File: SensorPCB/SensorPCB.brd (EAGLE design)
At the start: 36 x 66 mm, 31 parts, among them T1 33u

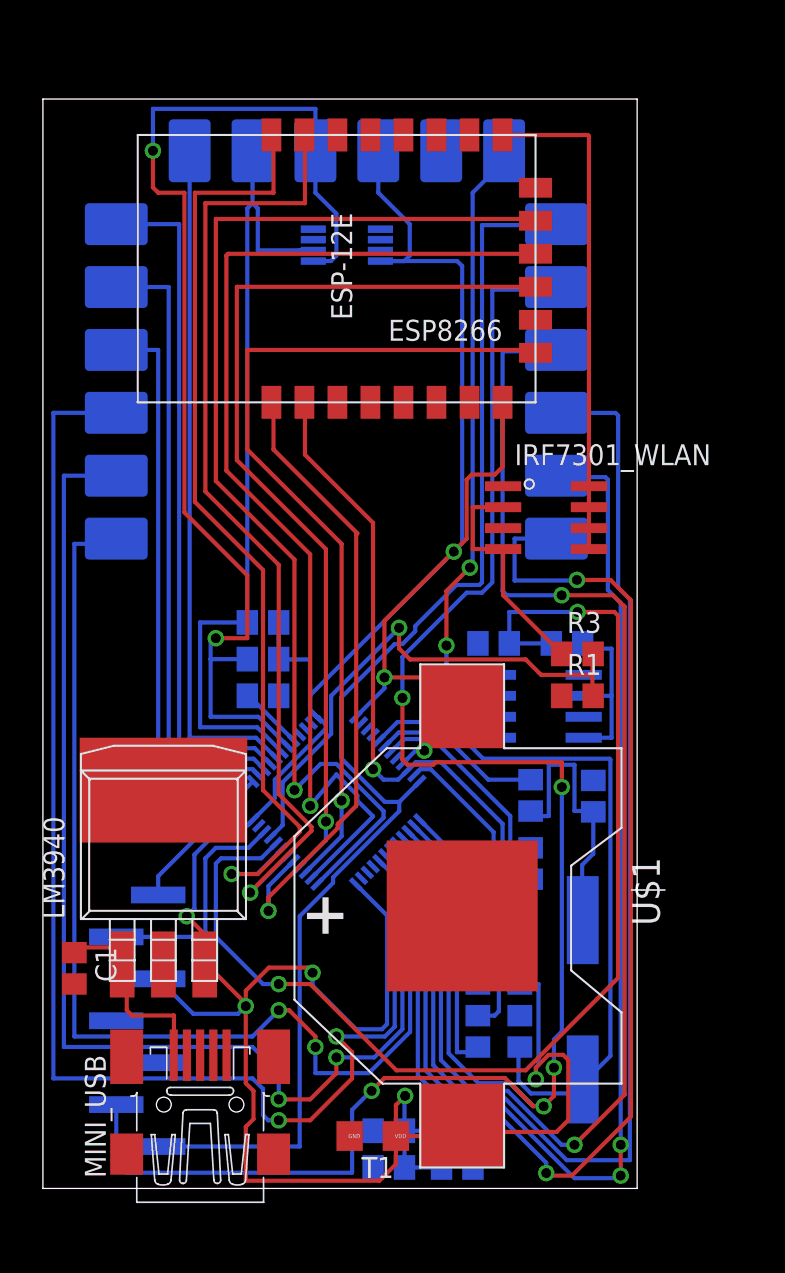
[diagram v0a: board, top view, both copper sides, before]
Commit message: start new board version
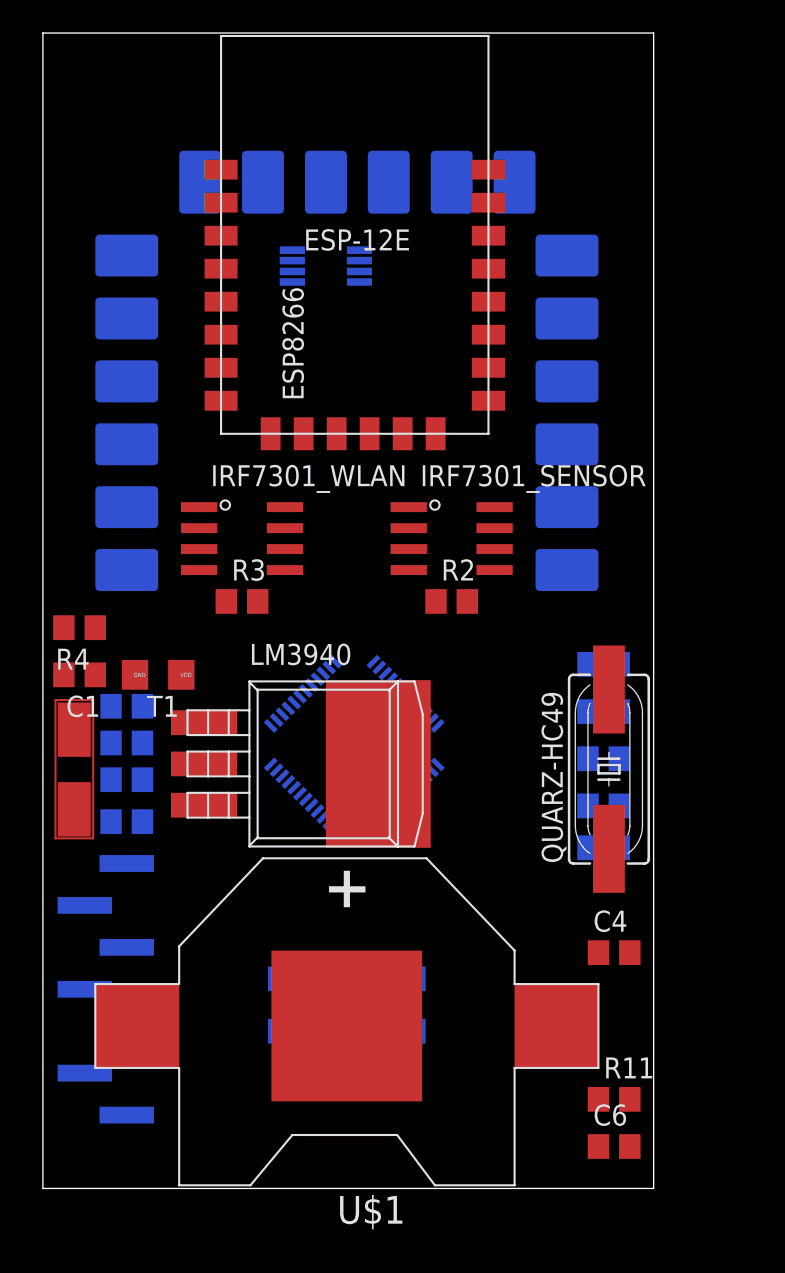
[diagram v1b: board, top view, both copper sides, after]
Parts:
- removed MINI_USB: MINI-USB-SCHIELD-32005-201, con-cypressindustries:32005-201
- added R4: 10k, rcl:R0805
- added U$2: 5V_POWER_SUPPLY, 5V_POWER_SUPPLY:5V_POWER_SUPPLY
- moved T1 30.8 mm to (6.99, 31.1)
- moved R1 27.8 mm to (5.08, 24.8), flipped to the bottom, turned to 180 degrees
- moved R6 24.7 mm to (5.08, 22.2)
- moved C6 21.3 mm to (34.6, 2.54), flipped to the top, turned to 0 degrees
- moved R10 20.9 mm to (34.0, 28.9)
- moved R3 20.6 mm to (12.1, 35.6)
- moved ESP8266 19.1 mm to (10.8, 45.7), turned to 0 degrees
- moved R11 19.1 mm to (34.6, 5.40), flipped to the top, turned to 0 degrees
- moved IRF7301_WLAN 18.5 mm to (12.1, 39.4)
- moved R7 18.2 mm to (34.0, 26.0), turned to 0 degrees
- moved C1 17.8 mm to (2.22, 31.1), turned to 180 degrees
- moved QUARZ-HC49 14.1 mm to (34.3, 25.4), flipped to the top, turned to 90 degrees
- moved C8 12.9 mm to (15.2, 9.53), turned to 0 degrees
- moved C10 12.9 mm to (34.0, 31.8), turned to 0 degrees
- moved C3 12.8 mm to (15.2, 12.7)
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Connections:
- removed net CH_PD_WLAN: ESP8266.3
- removed net D+: MINI_USB.3
- removed net D-: MINI_USB.2
- removed net ID: MINI_USB.4
- new net ADC: R7.2, R8.1, STM32L051C8T6.10
- new net CHPD: ESP8266.3, R4.1
- net +3V3: now also R4.2
- net +5V: now also U$2.MINUS; no longer MINI_USB.1
- net ADC_WLAN: no longer R7.2, R8.1, STM32L051C8T6.10
- net GND: now also U$2.PLUS; no longer MINI_USB.5
- net SPI2_MISO_WLAN: no longer STM32L051C8T6.27
- net SPI2_MOSI_WLAN: no longer STM32L051C8T6.28
- net SPI2_NSS_WLAN: no longer STM32L051C8T6.25
- net SPI2_SCK_WLAN: no longer STM32L051C8T6.26
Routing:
- net +3V3: track 204.4 -> 0.00 mm, vias 8 -> 0
- net USART2_RX_SENSOR: track 123.8 -> 0.00 mm, vias 5 -> 0
- net PA4: track 84.7 -> 0.00 mm, vias 2 -> 0
- net PB2: track 82.4 -> 0.00 mm, vias 2 -> 0
- net USART2_TX_SENSOR: track 80.1 -> 0.00 mm
- net PA5: track 78.3 -> 0.00 mm
- net PA7: track 75.8 -> 0.00 mm, vias 2 -> 0
- net PA6: track 75.1 -> 0.00 mm, vias 2 -> 0
- net PB1: track 73.9 -> 0.00 mm, vias 2 -> 0
- net SW_SENSOR: track 71.7 -> 0.00 mm, vias 2 -> 0
- net I2C1_SDA_SENSOR: track 71.7 -> 0.00 mm, vias 2 -> 0
- net SPI2_NSS_WLAN: track 69.3 -> 0.00 mm, vias 1 -> 0
- net PB0: track 69.0 -> 0.00 mm, vias 2 -> 0
- net SPI2_SCK_WLAN: track 65.5 -> 0.00 mm, vias 1 -> 0
- net USART1_TX_WLAN: track 59.4 -> 0.00 mm, vias 1 -> 0
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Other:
- board size 36 x 66 mm -> 37 x 70 mm
